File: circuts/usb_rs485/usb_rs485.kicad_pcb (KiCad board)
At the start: 2 copper layers, 47.8 x 40.2 mm, 66 parts, among them CON1 USB-MINI-B, IC1 SP3481CN, P2 CONN_2, U1 CP2102

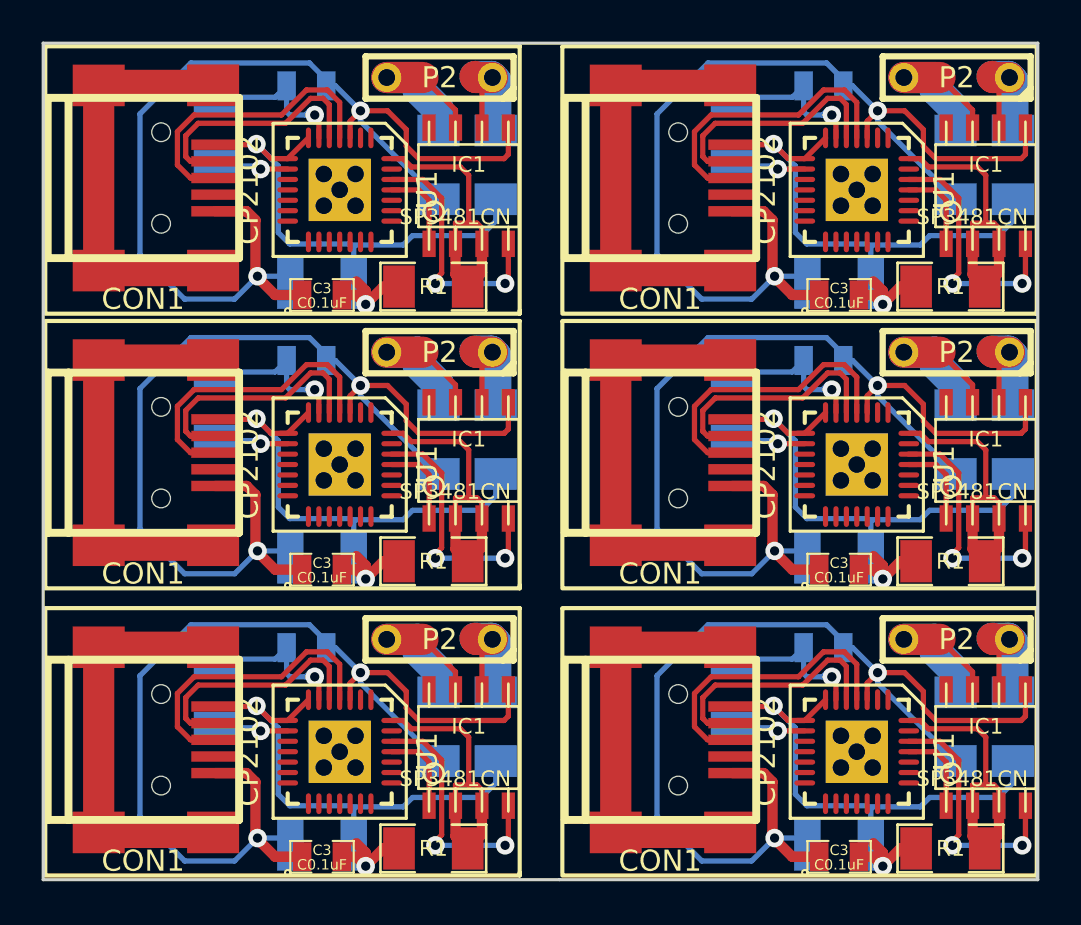
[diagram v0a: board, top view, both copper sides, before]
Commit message: For sending to iteadstudio.com
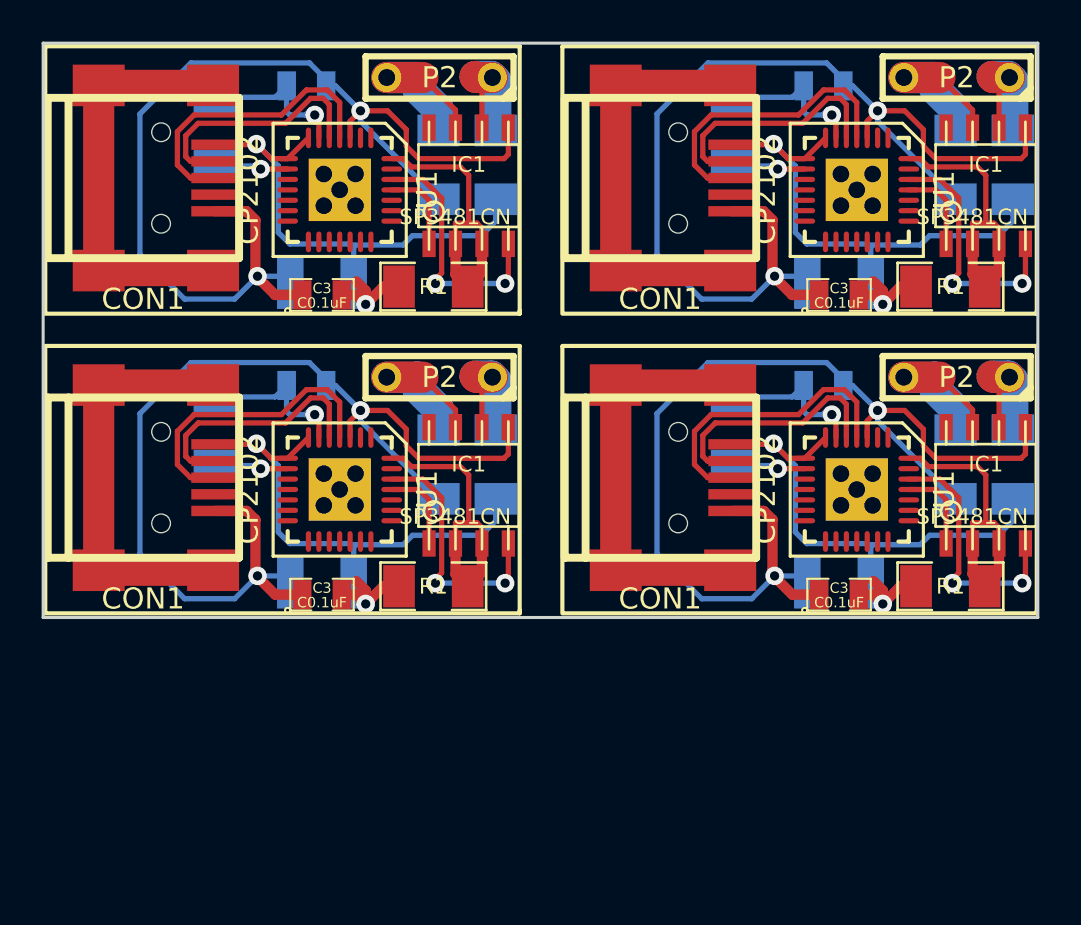
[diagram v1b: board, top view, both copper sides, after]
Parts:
- removed the C1 at (37.5, 29.1)
- removed the C1 at (12.7, 29.1)
- removed the C2 at (38.2, 38.5)
- removed the C2 at (13.4, 38.5)
- removed the C3 at (38.2, 39.1)
- removed the C3 at (13.4, 39.1)
- removed the CON1 at (29.7, 33.5)
- removed the CON1 at (4.82, 33.5)
- removed the IC1 at (45.3, 33.9)
- removed the IC1 at (20.4, 33.9)
- removed the P2 at (43.9, 28.6)
- removed the P2 at (19.1, 28.6)
- removed the R1 at (43.6, 38.7)
- removed the R1 at (18.8, 38.7)
- removed the R2 at (46.6, 32.9)
- removed the R2 at (21.8, 32.9)
- removed the R3 at (43.9, 32.9)
- removed the R3 at (19.0, 32.9)
- removed the R4 at (33.1, 31.2)
- removed the R4 at (8.25, 31.2)
- removed the U1 at (39.1, 34.0)
- removed the U1 at (14.2, 34.0)
- moved CON1 1.20 mm to (4.82, 20.9)
- moved CON1 1.20 mm to (29.7, 20.9)
- moved R1 1.20 mm to (18.8, 26.1)
- moved R1 1.20 mm to (43.6, 26.1)
- moved P2 1.20 mm to (19.1, 16.1)
- moved P2 1.20 mm to (43.9, 16.1)
- moved C1 1.20 mm to (12.7, 16.4)
- moved C1 1.20 mm to (37.5, 16.4)
- moved C2 1.20 mm to (13.4, 25.9)
- moved C2 1.20 mm to (38.2, 25.9)
- moved C3 1.20 mm to (13.4, 26.5)
- moved C3 1.20 mm to (38.2, 26.5)
- moved IC1 1.20 mm to (20.4, 21.2)
- moved IC1 1.20 mm to (45.3, 21.2)
- moved R2 1.20 mm to (21.8, 20.2)
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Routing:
- net GND: track 318.6 -> 212.4 mm, vias 12 -> 8
- net /VBUS: track 182.5 -> 121.7 mm, vias 12 -> 8
- net N-0000030: track 119.4 -> 79.6 mm
- net /D+: track 85.5 -> 57.0 mm
- net N-000002: track 84.5 -> 56.4 mm
- net N-000008: track 73.9 -> 49.3 mm, vias 12 -> 8
- net /D-: track 71.3 -> 47.5 mm
- net N-000005: track 56.3 -> 37.6 mm
- net /VDD: track 46.5 -> 31.0 mm, vias 6 -> 4
- net N-000004: track 41.7 -> 27.8 mm, vias 6 -> 4
- net /RX: track 24.6 -> 16.4 mm
- net N-0000010: track 21.4 -> 14.3 mm, vias 6 -> 4
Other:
- board size 47.8 x 40.2 mm -> 47.8 x 27.6 mm
